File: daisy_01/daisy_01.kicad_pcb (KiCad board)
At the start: 2 copper layers, 165.1 x 99.1 mm, 16 parts, among them J1 AudioInput, J2 AudioOutput1, J3 AudioOutput2, Q1 PN2222A, SW1 SW_SPST

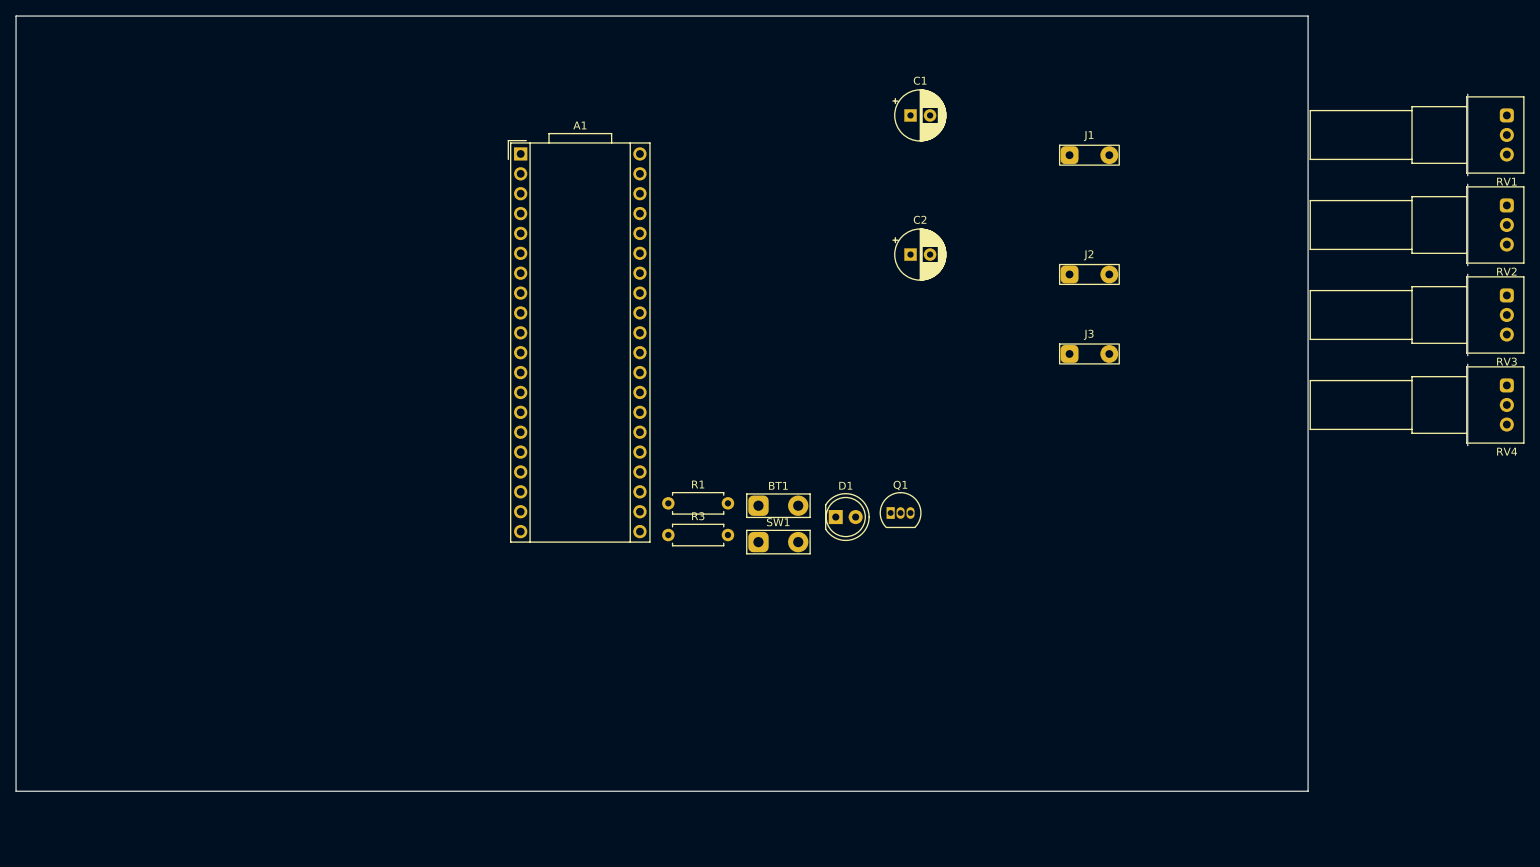
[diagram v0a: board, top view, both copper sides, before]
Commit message: update
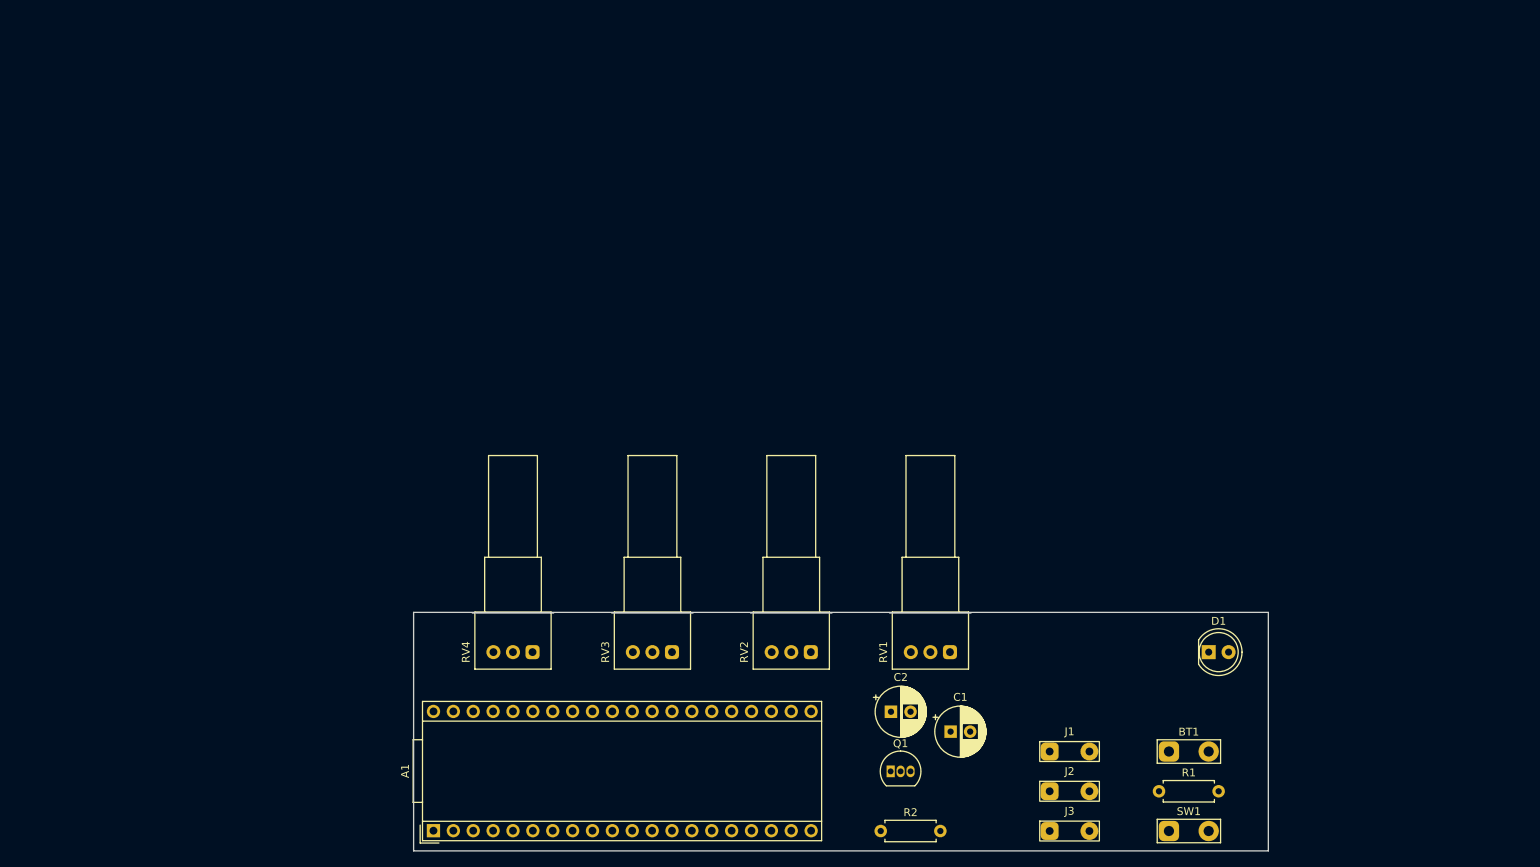
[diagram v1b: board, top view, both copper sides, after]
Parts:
- moved RV4 129.1 mm to (116.8, 106.7), turned to -90 degrees
- moved RV3 116.0 mm to (134.6, 106.7), turned to -90 degrees
- moved RV2 105.7 mm to (152.4, 106.7), turned to -90 degrees
- moved RV1 98.8 mm to (170.1, 106.7), turned to -90 degrees
- moved A1 87.2 mm to (104.1, 129.5), turned to 90 degrees
- moved C1 78.9 mm to (170.2, 116.8)
- moved J1 76.2 mm to (185.4, 119.4)
- moved R1 72.7 mm to (196.8, 124.5)
- moved J2 66.1 mm to (185.4, 124.5)
- moved SW1 64.1 mm to (198.1, 129.5)
- moved BT1 61.1 mm to (198.1, 119.4)
- moved J3 61.0 mm to (185.4, 129.5)
- moved C2 58.5 mm to (162.6, 114.3)
- moved D1 50.7 mm to (203.2, 106.7)
- moved R2 46.6 mm to (161.3, 129.5)
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- renumbered R3 to R2
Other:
- board size 165.1 x 99.1 mm -> 109.2 x 30.5 mm
